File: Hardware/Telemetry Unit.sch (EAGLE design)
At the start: 51 parts, among them IC1 MEGA128-A, IC2 FT232RL, J2 503182-1852, J3 10118193-0001LF, Q1 10MHz, U1 MPL3115A2, U2 AP65111A, U3 LSM6DS3

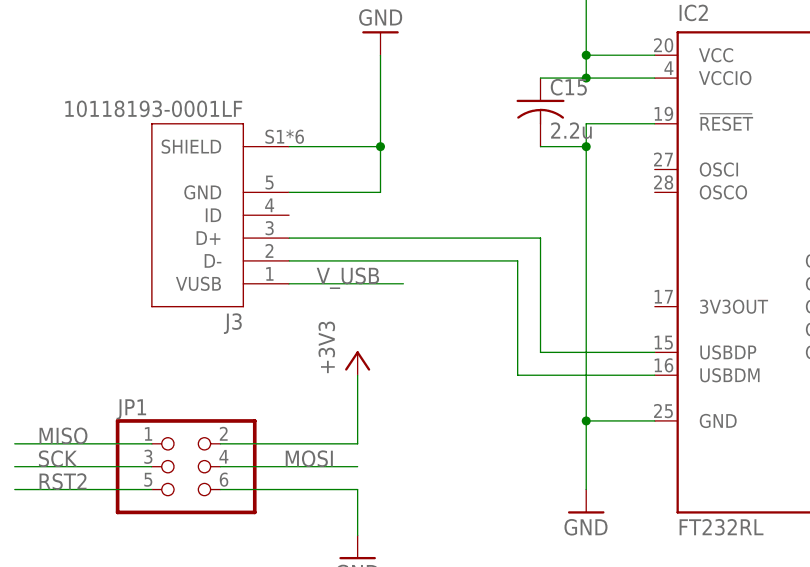
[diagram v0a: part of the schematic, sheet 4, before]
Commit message: Added fuse to usb
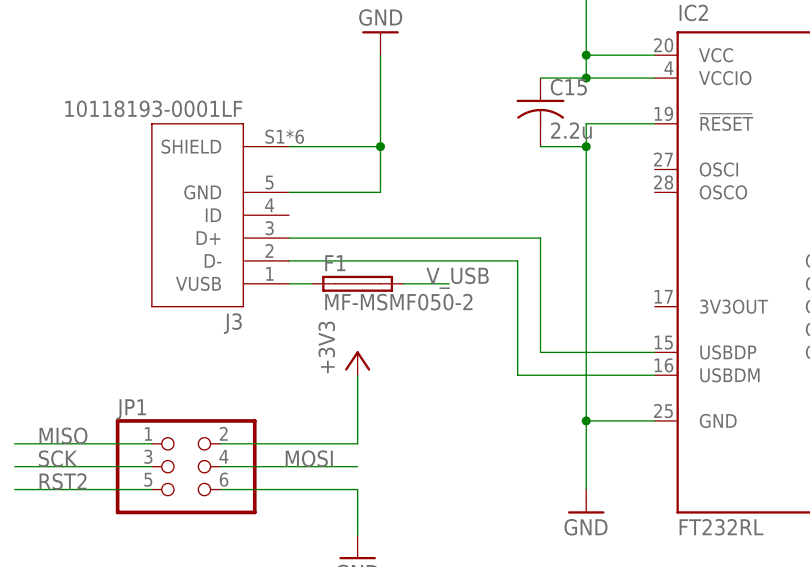
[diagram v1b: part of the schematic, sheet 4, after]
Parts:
- added F1: MF-MSMF050-2, MF-MSMF050-2:MF-MSMF050-2
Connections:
- new net N$22: F1.1, J3.VUSB
- net V_USB: now also F1.2; no longer J3.VUSB
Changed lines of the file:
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@@
 <?xml version="1.0" encoding="utf-8"?>
 <!DOCTYPE eagle SYSTEM "eagle.dtd">
-<eagle version="9.2.2">
+<eagle version="9.3.0">
 <drawing>
 <settings>
@@
 <part name="R15" library="resistor" library_urn="urn:adsk.eagle:library:348" deviceset="R-US_" device="R0603" package3d_urn="urn:adsk.eagle:package:23555/3" value="10k"/>
 <part name="R16" library="resistor" library_urn="urn:adsk.eagle:library:348" deviceset="R-US_" device="R0603" package3d_urn="urn:adsk.eagle:package:23555/3" value="10k"/>
+<part name="F1" library="MF-MSMF050-2" deviceset="MF-MSMF050-2" device=""/>
 </parts>
 <sheets>
@@
 <attribute name="VALUE" x="21.59" y="70.358" size="1.778" layer="96"/>
 </instance>
+<instance part="F1" gate="G$1" x="-55.88" y="50.8" smashed="yes">
+<attribute name="NAME" x="-59.69661875" y="52.19943125" size="1.781090625" layer="95"/>
+<attribute name="VALUE" x="-59.696859375" y="47.873740625" size="1.7812" layer="96"/>
+</instance>
 </instances>
 <busses>
@@
 </segment>
 </net>
-<net name="V_USB" class="0">
-<segment>
-<pinref part="J3" gate="G$1" pin="VUSB"/>
-<wire x1="-63.5" y1="50.8" x2="-50.8" y2="50.8" width="0.1524" layer="91"/>
-<label x="-53.34" y="50.8" size="1.778" layer="95" align="bottom-right"/>
-</segment>
-</net>
 <net name="N$11" class="0">
 <segment>
@@
 </segment>
 </net>
+<net name="N$22" class="0">
+<segment>
+<pinref part="J3" gate="G$1" pin="VUSB"/>
+<pinref part="F1" gate="G$1" pin="1"/>
+<wire x1="-63.5" y1="50.8" x2="-60.96" y2="50.8" width="0.1524" layer="91"/>
+</segment>
+</net>
+<net name="V_USB" class="0">
+<segment>
+<pinref part="F1" gate="G$1" pin="2"/>
+<wire x1="-50.8" y1="50.8" x2="-45.72" y2="50.8" width="0.1524" layer="91"/>
+<label x="-48.26" y="50.8" size="1.778" layer="95"/>
+</segment>
+</net>
